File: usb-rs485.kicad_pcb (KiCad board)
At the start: 4 copper layers, 27.5 x 35.8 mm, 33 parts, among them IC1 THVD2450VDRCR, J1 USB4110GFA, U12 DF52-4S-0.8H(21), U9 CP2102N-A02-GQFN24R

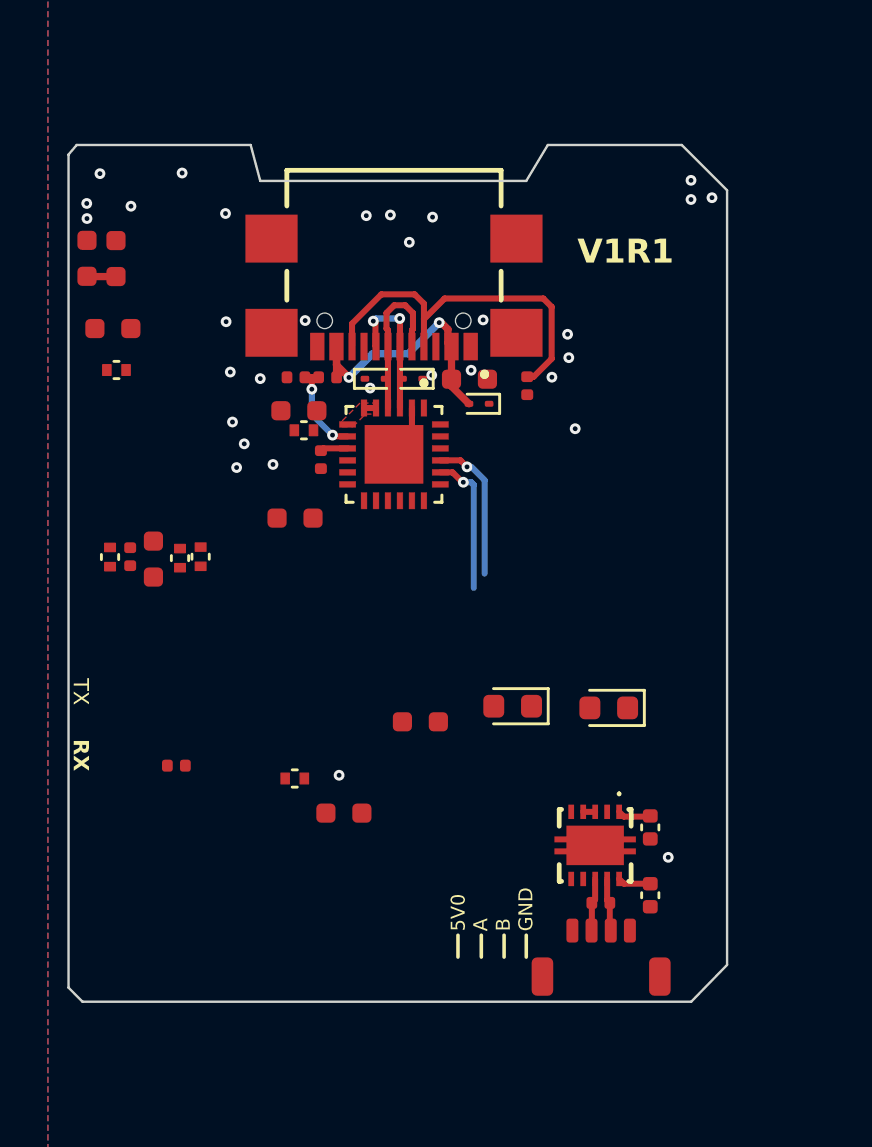
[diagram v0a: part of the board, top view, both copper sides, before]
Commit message: routing
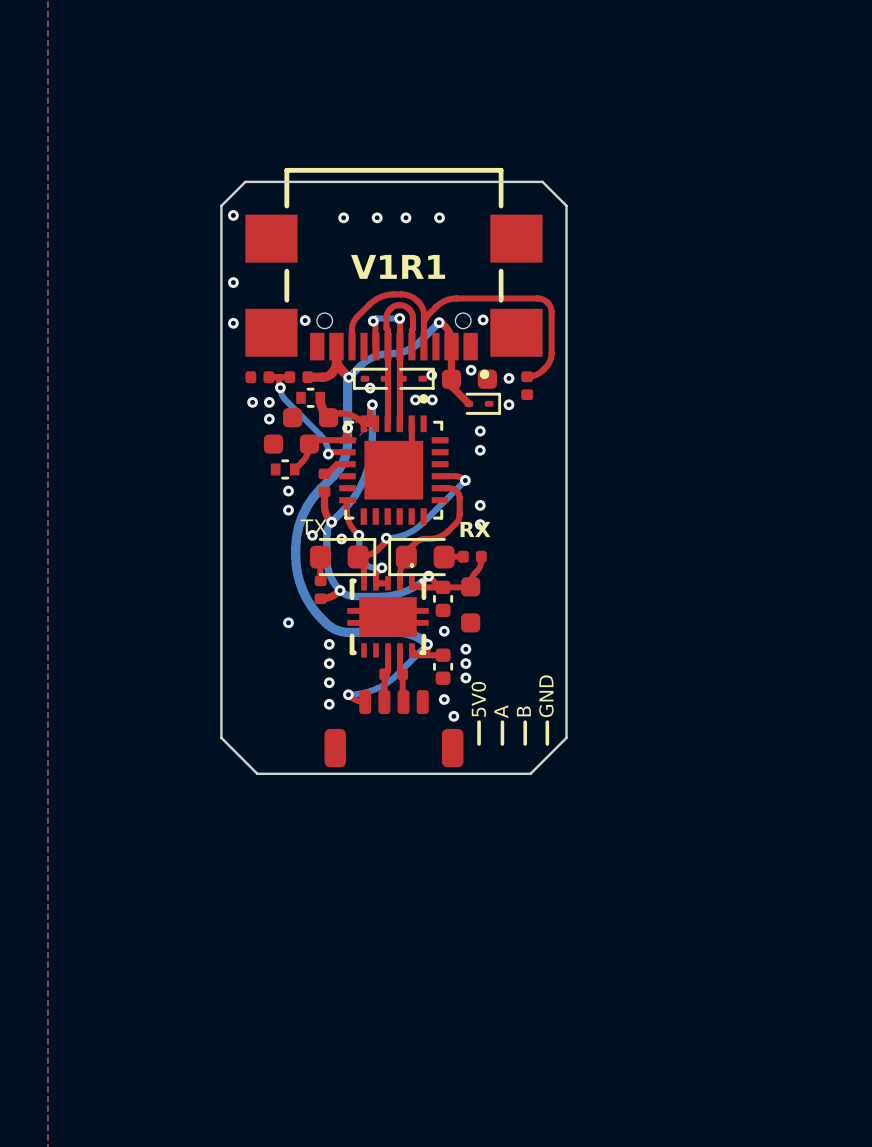
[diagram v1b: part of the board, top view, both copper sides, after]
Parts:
- removed C10, C19, C3, C6: 100nF, robot-cortex:C_0402_1005Metric
- removed C16, C17, C18: 4.7uF, robot-cortex:C_0603_1608Metric
- removed C2, C7: 10uF 0603, robot-cortex:C_0603_1608Metric
- C5: value 10uF 0603 -> 4.7uF 0603
- moved R2 14.3 mm to (146.4, 106.9), turned to 180 degrees
- moved D5 12.9 mm to (140.8, 106.9)
- moved C1 12.9 mm to (145.2, 108.6)
- moved IC1 12.9 mm to (142.9, 109.4)
- moved C28 12.9 mm to (145.2, 111.5)
- moved U12 12.9 mm to (143.1, 112.9)
- moved R19 12.9 mm to (143.1, 111.8)
- moved C9 10.2 mm to (146.3, 108.9), turned to -90 degrees
- moved R3 9.49 mm to (140.1, 108.3), turned to 90 degrees
- moved C8 8.06 mm to (139.6, 100.2), turned to 180 degrees
- moved D4 7.21 mm to (144.4, 106.9), turned to 0 degrees
- moved C5 4.24 mm to (139.6, 101.1), turned to 180 degrees
- moved C21 1.81 mm to (138.6, 103.2)
- moved R8 1.51 mm to (137.5, 99.4)
- moved C20 1.42 mm to (138.8, 102.2)
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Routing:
- net /VUSB: track 12.8 -> 40.0 mm, vias 2 -> 5
- net +3V3: track 3.11 -> 23.3 mm, vias 0 -> 4
- net /DE: track 0.50 -> 4.87 mm, vias 0 -> 2
- net /TX: track 6.09 -> 7.97 mm, vias 1 -> 2
- net /CP2102N/CP210x_VBUS: track 4.27 -> 6.11 mm
- net Net-(D5-A): track 0.00 -> 0.99 mm
- net Net-(D4-A): track 0.00 -> 0.81 mm
- net /CP2102N/D+: track 6.01 -> 6.67 mm
- net /CP2102N/D-: track 6.78 -> 7.35 mm
- net /RX: track 5.91 -> 5.98 mm, vias 1 -> 0
- net GND: vias 31 -> 38
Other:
- board size 27.5 x 35.8 mm -> 14.4 x 24.7 mm
